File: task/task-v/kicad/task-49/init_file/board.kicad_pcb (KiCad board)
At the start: 2 copper layers, 100 x 100 mm, 4 parts

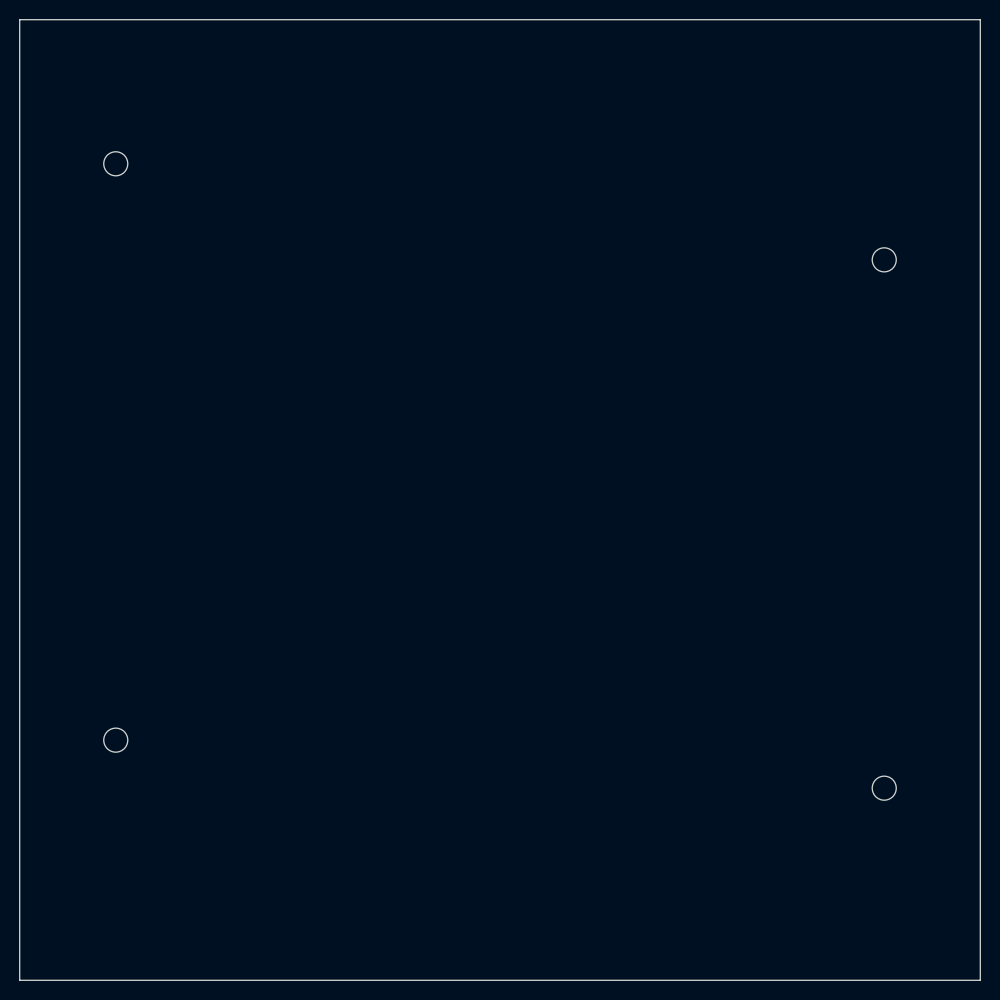
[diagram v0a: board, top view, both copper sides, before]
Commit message: Refine engineering task metadata and instructions
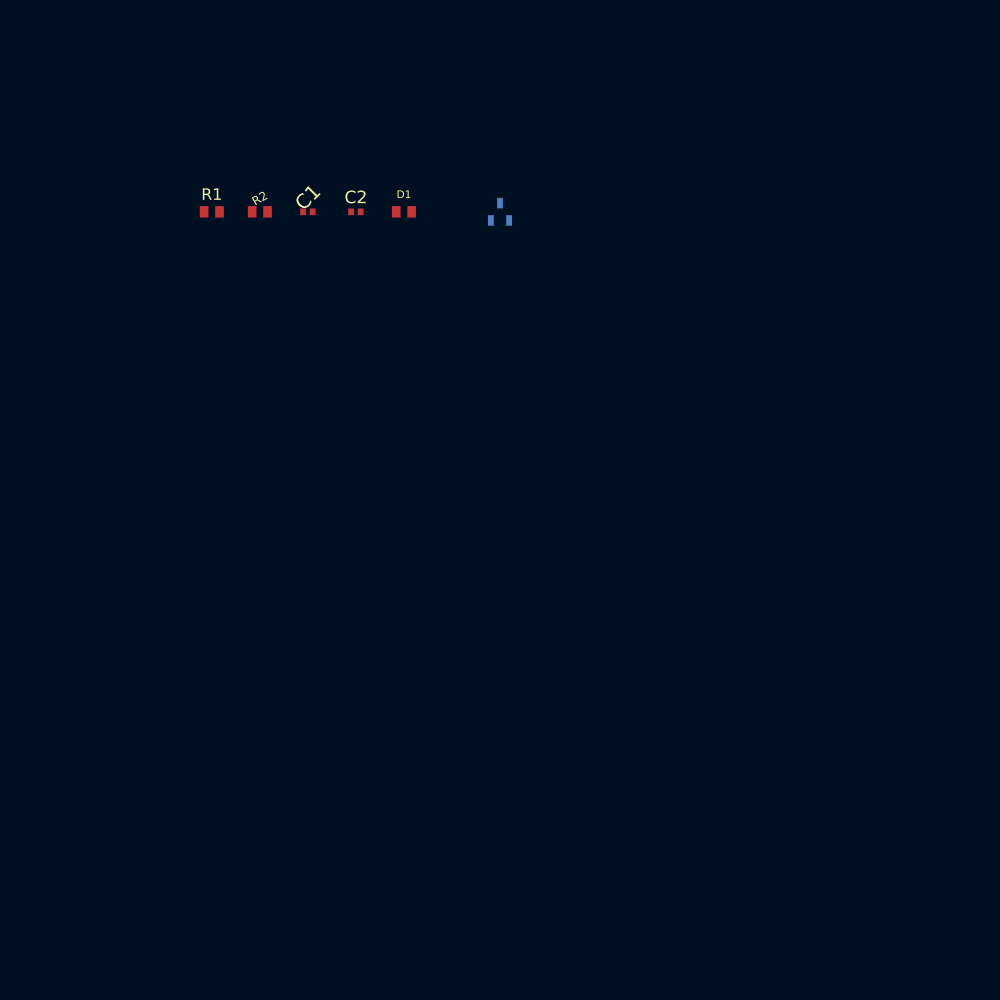
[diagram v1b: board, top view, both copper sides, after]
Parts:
- removed ? (x4): , MountingHole:MountingHole_2.75mm_M2.5
- added C1: 100nF, Capacitor_SMD:C_0402_1005Metric, F.Cu at (30.0, 20.0)
- added C2: 10uF, Capacitor_SMD:C_0402_1005Metric, F.Cu at (35.0, 20.0)
- added D1: LED_RED, LED_SMD:LED_0603_1608Metric, F.Cu at (40.0, 20.0)
- added Q1: MMBT3904, Package_TO_SOT_SMD:SOT-23, F.Cu at (50.0, 20.0)
- added R1: 10k, Resistor_SMD:R_0603_1608Metric, F.Cu at (20.0, 20.0)
- added R2: 4k7, Resistor_SMD:R_0603_1608Metric, F.Cu at (25.0, 20.0)
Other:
- board outline removed
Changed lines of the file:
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@@
     (0 "F.Cu" signal)
     (31 "B.Cu" signal)
+    (36 "B.SilkS" user "B.Silkscreen")
+    (37 "F.SilkS" user "F.Silkscreen")
+    (38 "B.Mask" user)
+    (39 "F.Mask" user)
     (44 "Edge.Cuts" user)
+    (46 "B.CrtYd" user "B.Courtyard")
+    (47 "F.CrtYd" user "F.Courtyard")
+    (48 "B.Fab" user)
+    (49 "F.Fab" user)
   )
   (setup
     (pad_to_mask_clearance 0.1)
-    (allow_soldermask_bridges_in_footprints no)
   )
   (net 0 "")
-  (net 1 "GND")
-  (net 2 "VCC")
-  ; 4 non-plated mounting holes (np_thru_hole)
-  ; H1 at (10,15): Y=15 < analog_midline=50 — lowest Y, stays isolated (analog side)
-  (footprint "MountingHole:MountingHole_2.75mm_M2.5" (layer "F.Cu") (at 10 15)
-    (reference "H1") (value "MountingHole")
-    (attr through_hole)
-    (pad "" np_thru_hole circle (at 0 0) (size 2.5 2.5) (drill 2.5)
-      (layers "F.Cu" "B.Cu" "F.Mask" "B.Mask"))
+  (net 1 "VCC")
+  (net 2 "GND")
+  (net 3 "SIG_A")
+  (net 4 "SIG_B")
+  (footprint "Resistor_SMD:R_0603_1608Metric" (layer "F.Cu")
+    (at 20 20)
+    (fp_text reference "R1" (at 0 -1.8 0) (layer "F.SilkS")
+      (effects (font (size 1.2 1.2) (thickness 0.18)))
+    )
+    (fp_text value "10k" (at 0 1.8 0) (layer "F.Fab")
+      (effects (font (size 1 1) (thickness 0.15)))
+    )
+    (pad "1" smd rect (at -0.8 0) (size 0.9 1.2) (layers "F.Cu" "F.Paste" "F.Mask") (net 1 "VCC"))
+    (pad "2" smd rect (at 0.8 0) (size 0.9 1.2) (layers "F.Cu" "F.Paste" "F.Mask") (net 2 "GND"))
   )
-  ; H2 at (90,25): Y=25 < 50 but higher Y than H1 — will become plated GND
-  (footprint "MountingHole:MountingHole_2.75mm_M2.5" (layer "F.Cu") (at 90 25)
-    (reference "H2") (value "MountingHole")
-    (attr through_hole)
-    (pad "" np_thru_hole circle (at 0 0) (size 2.5 2.5) (drill 2.5)
-      (layers "F.Cu" "B.Cu" "F.Mask" "B.Mask"))
+  (footprint "Resistor_SMD:R_0603_1608Metric" (layer "F.Cu")
+    (at 25 20)
+    (fp_text reference "R2" (at 0 -1.4 30) (layer "F.SilkS")
+      (effects (font (size 0.9 0.9) (thickness 0.12)))
+    )
+    (fp_text value "4k7" (at 0 1.8 0) (layer "F.Fab")
+      (effects (font (size 1 1) (thickness 0.15)))
+    )
+    (pad "1" smd rect (at -0.8 0) (size 0.9 1.2) (layers "F.Cu" "F.Paste" "F.Mask") (net 1 "VCC"))
+    (pad "2" smd rect (at 0.8 0) (size 0.9 1.2) (layers "F.Cu" "F.Paste" "F.Mask") (net 3 "SIG_A"))
   )
-  ; H3 at (10,75): Y=75 > 50 — will become plated GND
-  (footprint "MountingHole:MountingHole_2.75mm_M2.5" (layer "F.Cu") (at 10 75)
-    (reference "H3") (value "MountingHole")
-    (attr through_hole)
-    (pad "" np_thru_hole circle (at 0 0) (size 2.5 2.5) (drill 2.5)
-      (layers "F.Cu" "B.Cu" "F.Mask" "B.Mask"))
+  (footprint "Capacitor_SMD:C_0402_1005Metric" (layer "F.Cu")
+    (at 30 20)
+    (fp_text reference "C1" (at 0 -1.5 45) (layer "F.SilkS")
+      (effects (font (size 1.5 1.5) (thickness 0.2)))
+    )
+    (fp_text value "100nF" (at 0 1.5 0) (layer "F.Fab")
+      (effects (font (size 1 1) (thickness 0.15)))
+    )
+    (pad "1" smd rect (at -0.5 0) (size 0.6 0.7) (layers "F.Cu" "F.Paste" "F.Mask") (net 1 "VCC"))
+    (pad "2" smd rect (at 0.5 0) (size 0.6 0.7) (layers "F.Cu" "F.Paste" "F.Mask") (net 2 "GND"))
   )
-  ; H4 at (90,80): Y=80 > 50 — will become plated GND
-  (footprint "MountingHole:MountingHole_2.75mm_M2.5" (layer "F.Cu") (at 90 80)
-    (reference "H4") (value "MountingHole")
-    (attr through_hole)
-    (pad "" np_thru_hole circle (at 0 0) (size 2.5 2.5) (drill 2.5)
-      (layers "F.Cu" "B.Cu" "F.Mask" "B.Mask"))
+  (footprint "Capacitor_SMD:C_0402_1005Metric" (layer "F.Cu")
+    (at 35 20)
+    (fp_text reference "C2" (at 0 -1.5 0) (layer "F.SilkS")
+      (effects (font (size 1.3 1.3) (thickness 0.17)))
+    )
+    (fp_text value "10uF" (at 0 1.5 0) (layer "F.Fab")
+      (effects (font (size 1 1) (thickness 0.15)))
+    )
+    (pad "1" smd rect (at -0.5 0) (size 0.6 0.7) (layers "F.Cu" "F.Paste" "F.Mask") (net 3 "SIG_A"))
+    (pad "2" smd rect (at 0.5 0) (size 0.6 0.7) (layers "F.Cu" "F.Paste" "F.Mask") (net 2 "GND"))
   )
-  (gr_rect (start 0 0) (end 100 100) (layer "Edge.Cuts") (width 0.1))
+  (footprint "LED_SMD:LED_0603_1608Metric" (layer "F.Cu")
+    (at 40 20)
+    (fp_text reference "D1" (at 0 -1.8 0) (layer "F.SilkS")
+      (effects (font (size 0.8 0.8) (thickness 0.1)))
+    )
+    (fp_text value "LED_RED" (at 0 1.8 0) (layer "F.Fab")
+      (effects (font (size 1 1) (thickness 0.15)))
+    )
+    (pad "1" smd rect (at -0.8 0) (size 0.9 1.2) (layers "F.Cu" "F.Paste" "F.Mask") (net 2 "GND"))
+    (pad "2" smd rect (at 0.8 0) (size 0.9 1.2) (layers "F.Cu" "F.Paste" "F.Mask") (net 4 "SIG_B"))
+  )
+  (footprint "Package_TO_SOT_SMD:SOT-23" (layer "F.Cu")
+    (at 50 20)
+    (fp_text reference "Q1" (at 0 -3.0 0) (layer "B.SilkS")
+      (effects (font (size 1.0 1.0) (thickness 0.15)))
+    )
+    (fp_text value "MMBT3904" (at 0 3.0 0) (layer "B.Fab")
+      (effects (font (size 1 1) (thickness 0.15)))
+    )
+    (pad "1" smd rect (at -0.95 0.9) (size 0.6 1.1) (layers "B.Cu" "B.Paste" "B.Mask") (net 2 "GND"))
+    (pad "2" smd rect (at 0.95 0.9) (size 0.6 1.1) (layers "B.Cu" "B.Paste" "B.Mask") (net 4 "SIG_B"))
+    (pad "3" smd rect (at 0 -0.9) (size 0.6 1.1) (layers "B.Cu" "B.Paste" "B.Mask") (net 1 "VCC"))
+  )
 )
